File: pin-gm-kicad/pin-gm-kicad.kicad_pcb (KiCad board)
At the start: 2 copper layers, 38 parts, among them U1 LM358, U2 TL072

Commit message: kis haladás
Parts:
- moved C4 219.3 mm to (28.0, 65.0)
- moved C7 216.1 mm to (36.5, 76.0), turned to 0 degrees
- moved L1 211.8 mm to (54.0, 80.0)
- moved C5 205.5 mm to (36.5, 73.0), turned to 0 degrees
- moved R11 129.1 mm to (205.2, 45.1)
- moved R2 129.1 mm to (190.9, 54.6)
- moved R3 129.1 mm to (188.5, 61.1)
- moved R5 129.1 mm to (205.2, 41.9)
- moved R8 129.1 mm to (214.4, 36.0)
- moved C1 129.1 mm to (176.5, 61.1)
- moved C11 129.1 mm to (208.4, 36.9)
- moved C12 129.1 mm to (204.7, 33.1)
- moved C14 129.1 mm to (199.2, 45.2)
- moved C15 129.1 mm to (191.0, 50.8)
- moved C2 129.1 mm to (199.2, 41.9)
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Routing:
- net GND: track 0.54 -> 0.00 mm
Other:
- board outline added: 70 x 84 mm

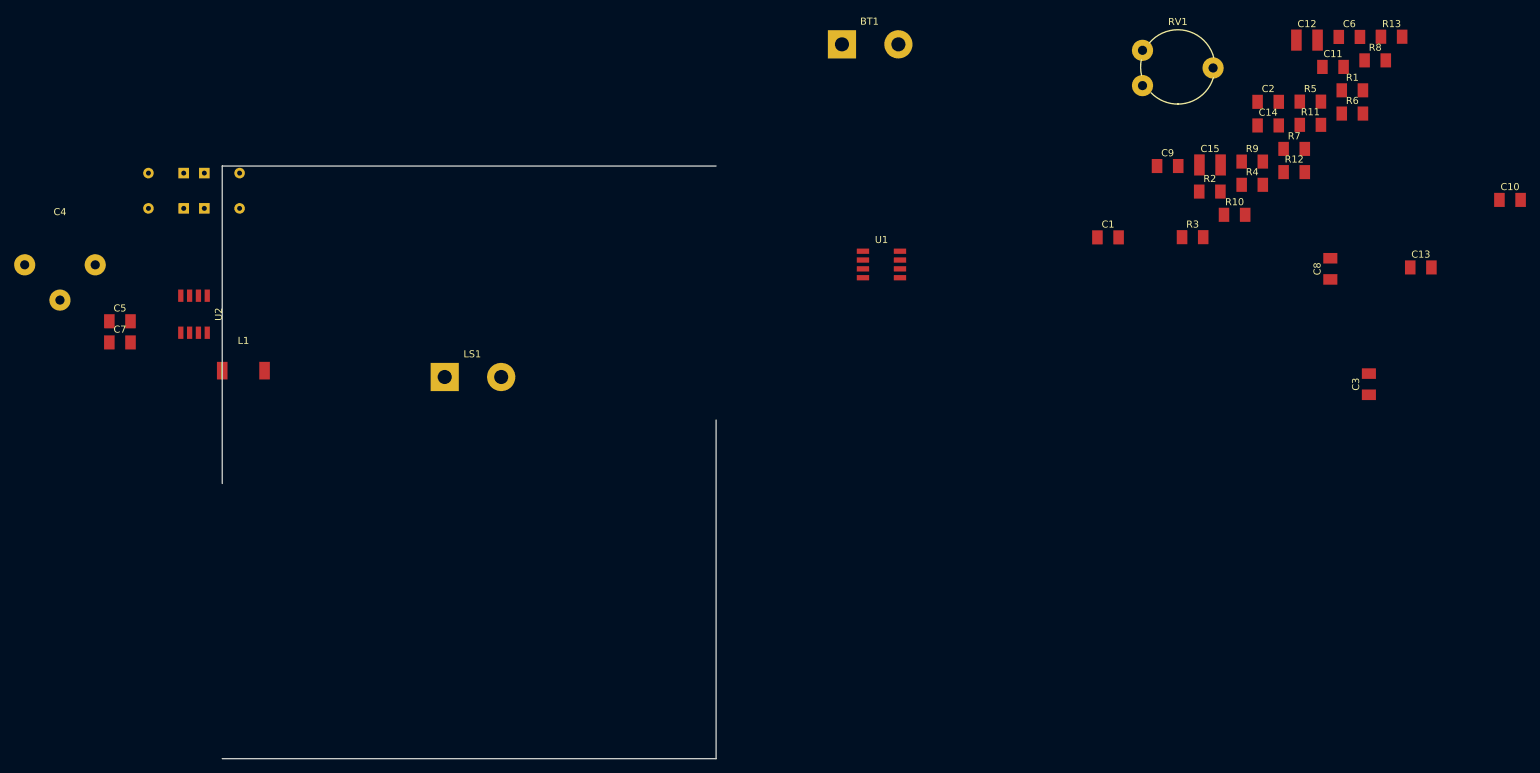
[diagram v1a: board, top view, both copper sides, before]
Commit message: kb elhelyezve
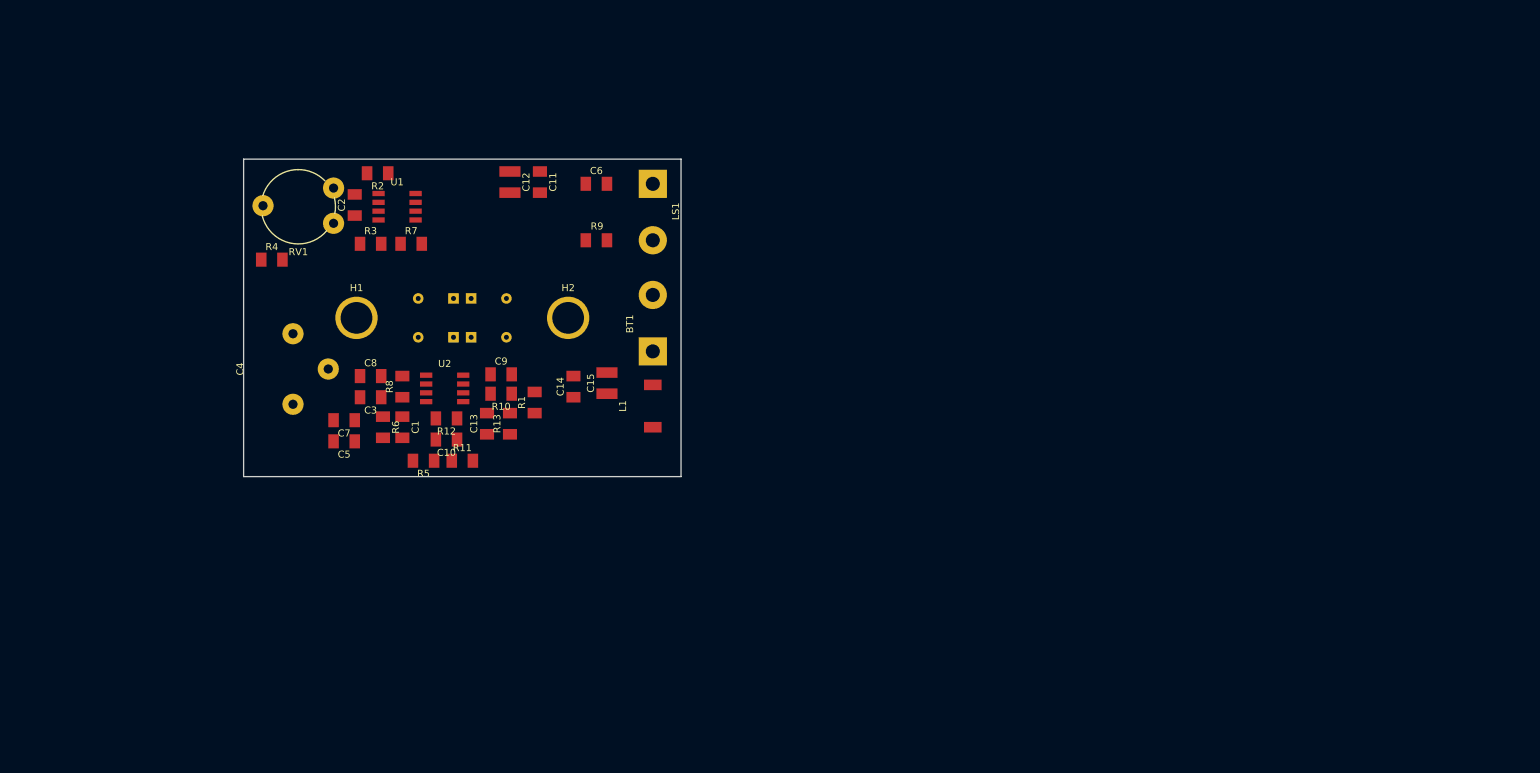
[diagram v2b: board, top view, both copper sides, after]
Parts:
- added H1: MountingHole_Pad, Homemade:Mounting_Hole_Dhole4mm_homemade, F.Cu at (70.0, 72.5)
- added H2: MountingHole_Pad, Homemade:Mounting_Hole_Dhole4mm_homemade, F.Cu at (100.0, 72.5)
- moved C10 154.5 mm to (82.8, 89.8), turned to 180 degrees
- moved R8 145.4 mm to (76.5, 82.2), turned to 90 degrees
- moved R6 144.4 mm to (73.8, 88.0), turned to -90 degrees
- moved C3 141.5 mm to (72.0, 83.8), turned to 180 degrees
- moved R4 139.4 mm to (58.0, 64.2)
- moved C8 136.9 mm to (72.0, 80.8), turned to 0 degrees
- moved R13 136.5 mm to (91.8, 87.5), turned to 90 degrees
- moved R5 135.6 mm to (79.5, 92.8), turned to 180 degrees
- moved C13 134.2 mm to (88.5, 87.5), turned to 90 degrees
- moved C2 130.3 mm to (69.8, 56.5), turned to 90 degrees
- moved R11 129.3 mm to (85.0, 92.8)
- moved R7 125.9 mm to (77.8, 62.0)
- moved R12 125.1 mm to (82.8, 86.8), turned to 180 degrees
- moved R1 124.1 mm to (95.2, 84.5), turned to 90 degrees
- moved R2 118.0 mm to (73.0, 52.0), turned to 180 degrees
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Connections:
- R8 pad 2: Net-(R8-Pad2) -> Net-(C8-Pad2)
- U2 pad 1: Net-(R8-Pad2) -> Net-(C8-Pad2)
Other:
- board size 70 x 84 mm -> 62 x 45 mm
